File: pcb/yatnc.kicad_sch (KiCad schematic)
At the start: 36 parts, among them J1 Conn_01x10_Socket, J3 Conn_01x02_Socket, J4 Conn_01x03_Pin, J5 DFR0570, J6 Conn_01x13_Socket, J7 Conn_01x13_Socket, Q1 BC547, SW1 SW_Push, U1 MAX3232

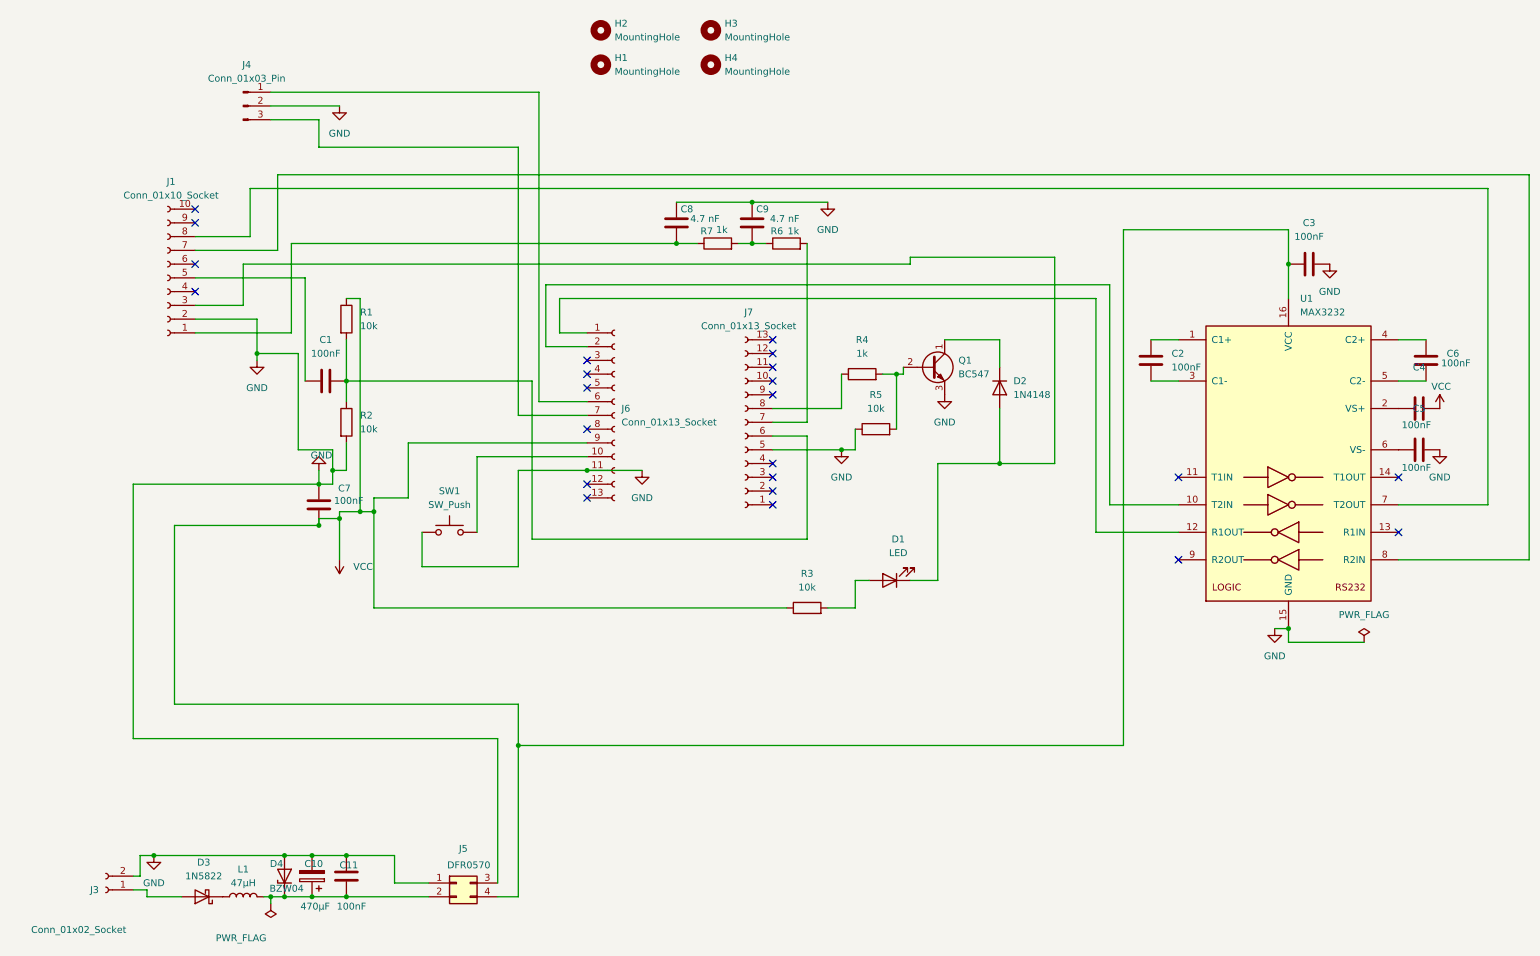
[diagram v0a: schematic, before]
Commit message: first part of changes after review
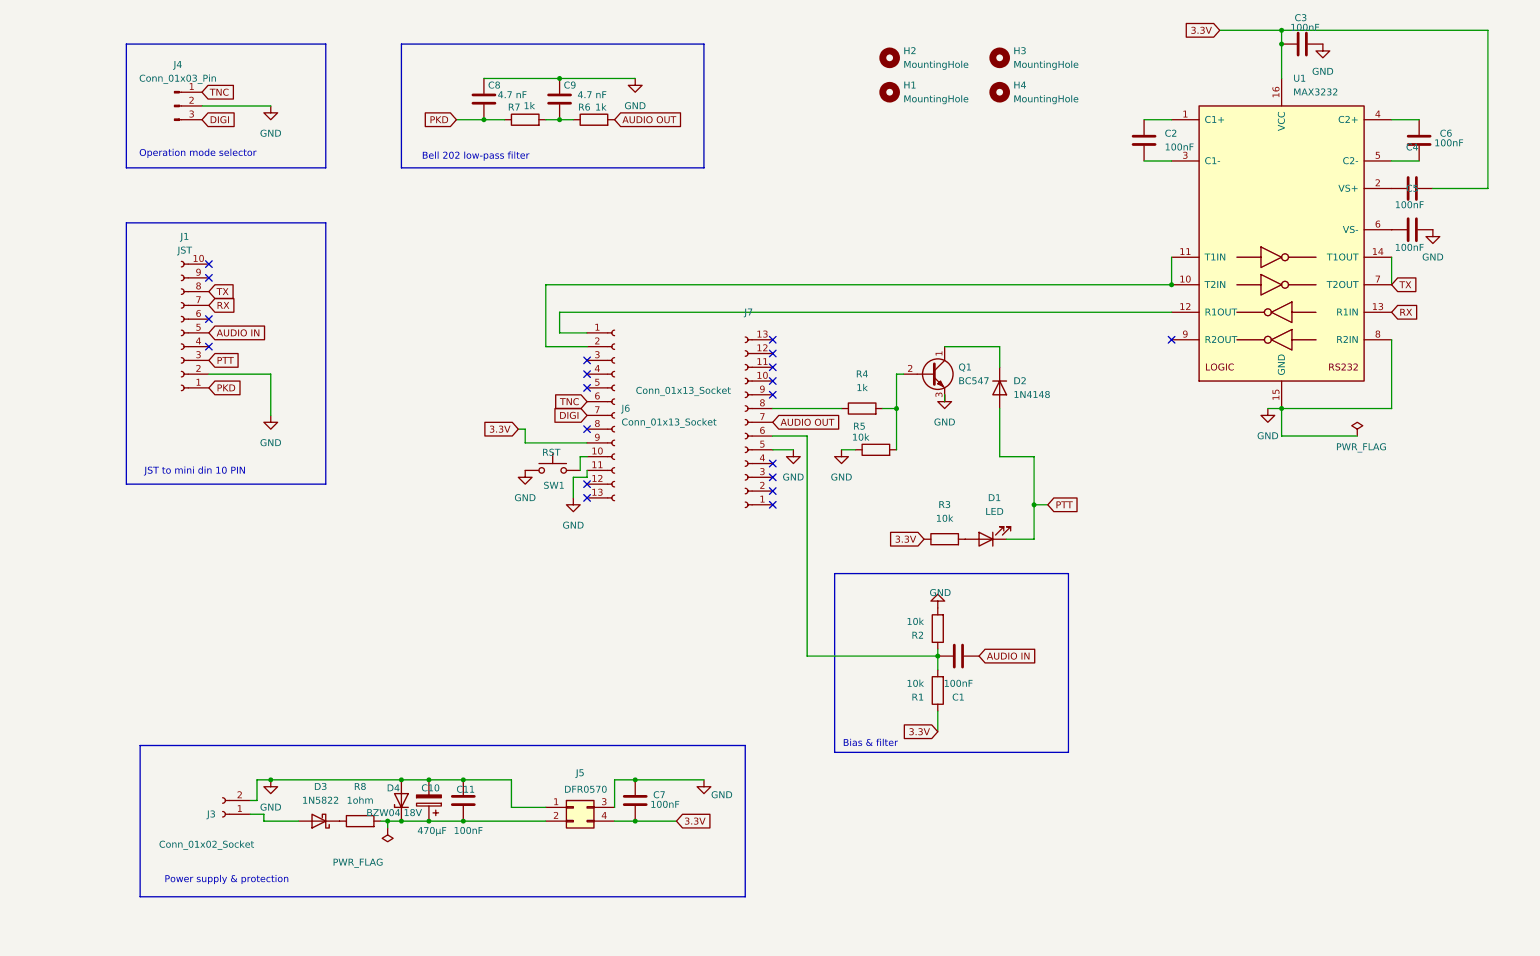
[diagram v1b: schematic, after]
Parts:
- removed L1: 47µH, Inductor_THT:L_Radial_D7.0mm_P3.00mm, symbol Device:L
- added R8: 1ohm, Resistor_THT:R_Axial_DIN0207_L6.3mm_D2.5mm_P10.16mm_Horizontal, symbol Device:R
- D4: value BZW04 -> BZW04 18V
- J1: value Conn_01x10_Socket -> JST
- SW1: value SW_Push -> RST
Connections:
- net GND: now also U1.8 (R2IN)
- net AUDIO OUT: now reaches J7.7 (Pin_7), R6.2
- net PTT: now reaches D1.1 (K), D2.2 (A), J1.3 (Pin_3)
- net PKD: now reaches C8.2, J1.1 (Pin_1), R7.1
- net AUDIO IN: now reaches C1.1, J1.5 (Pin_5)
- net RX: now reaches J1.7 (Pin_7)
- net RX: now also U1.13 (R1IN); no longer U1.8 (R2IN)
- net TX: now reaches J1.8 (Pin_8), U1.7 (T2OUT)
- net TX: now also U1.14 (T1OUT)
- net TNC: now reaches J4.1 (Pin_1), J6.6 (Pin_6)
- net DIGI: now reaches J4.3 (Pin_3), J6.7 (Pin_7)
- net at C10.1, C11.2, D4.1 (K)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: now also R8.2
- net at J6.2 (Pin_2), U1.10 (T2IN): now also U1.11 (T1IN)
- net at D3.1 (K): now also R8.1
- net VCC renamed 3.3V
- no-connect marks 23 -> 20
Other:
- note added: "Bell 202 low-pass filter"
- note added: "Bias & filter"
- note added: "JST to mini din 10 PIN"
- note added: "Operation mode selector"
- note added: "Power supply & protection"
- moved on the sheet: C1, C10, C11, C2, C3, C4, C5, C6, C7, C8, C9, D1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
